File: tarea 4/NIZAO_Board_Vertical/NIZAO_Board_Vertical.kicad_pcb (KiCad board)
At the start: 2 copper layers, 36.2 x 39.5 mm, 3 parts

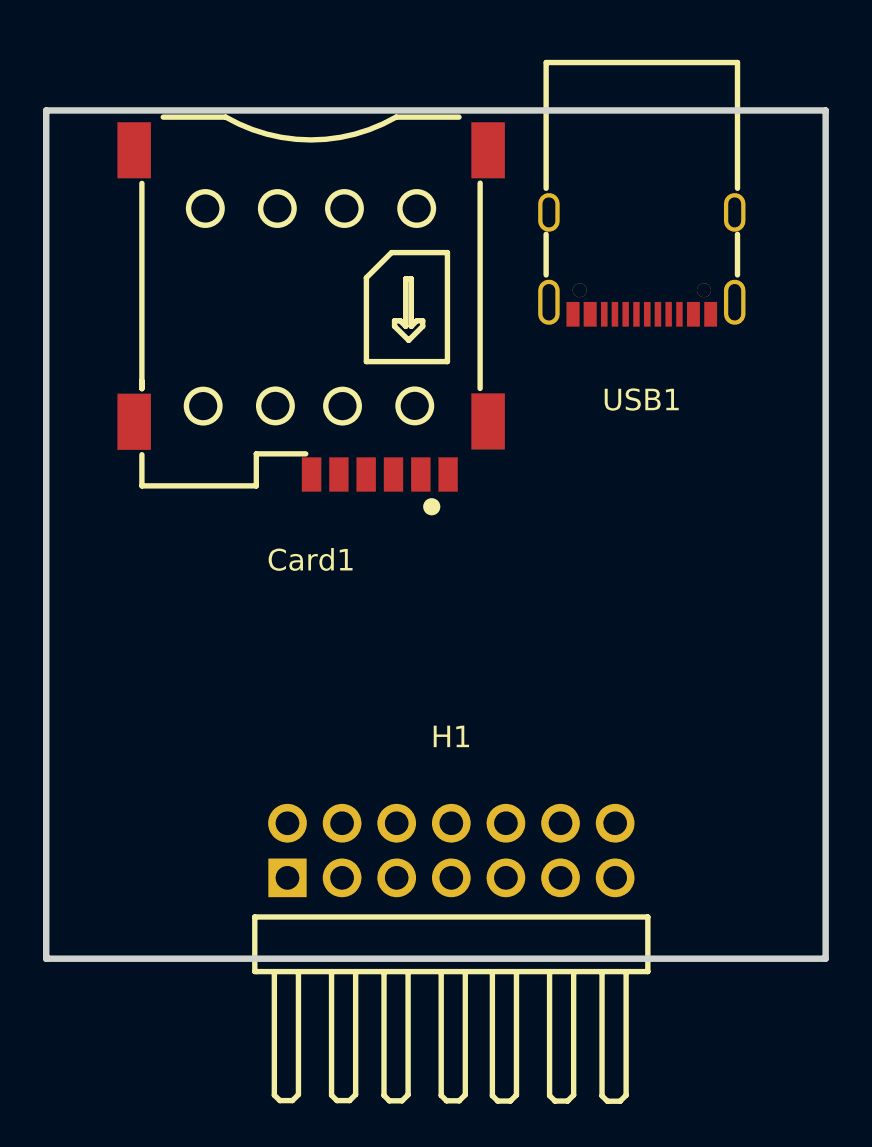
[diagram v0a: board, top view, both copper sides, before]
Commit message: actualizacion
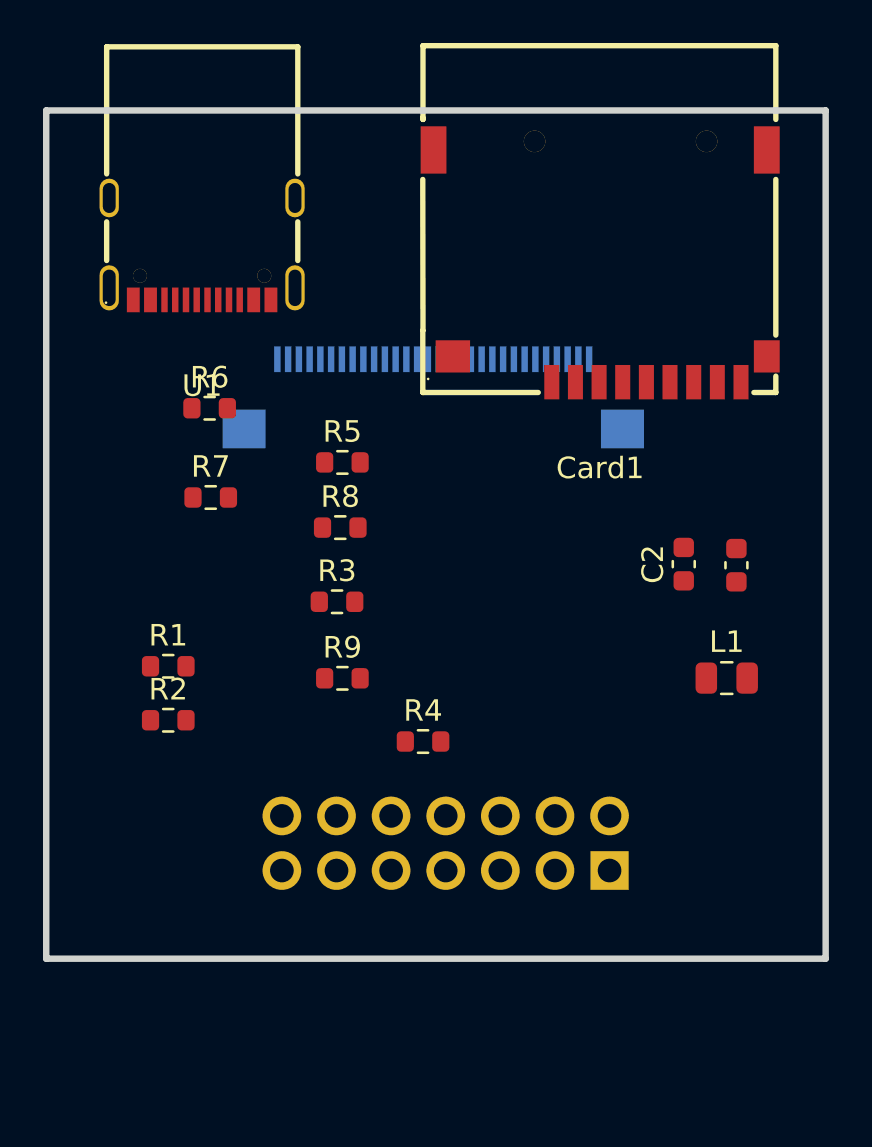
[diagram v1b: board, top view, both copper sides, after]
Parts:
- removed H1: PZ254R-12-14P, easyeda2kicad:HDR-TH_14P-P2.54-H-M-R2-C7-S2.54
- removed USB1: LCK-TCF809-L117YL-G1, easyeda2kicad:USB-C-SMD_LCK-TCF809-L117YL-G1
- added C1: 47uF, Capacitor_SMD:C_0603_1608Metric, F.Cu at (158.2, 102.2)
- added C2: 100nF, Capacitor_SMD:C_0603_1608Metric, F.Cu at (155.8, 102.1)
- added FPC1: FPC-05FB-30PH20, EasyEDA:FPC-SMD_30P-P0.50_FPC-05FB-30PH20, B.Cu at (144.1, 94.2)
- added J1: PZ254R-12-14P, EasyEDA:HDR-TH_14P-P2.54-H-M-R2-C7-S2.54, B.Cu at (144.7, 115.1)
- added L1: 600 Ohm, Capacitor_SMD:C_0805_2012Metric, F.Cu at (157.8, 107.4)
- added R1: 5.1k, Resistor_SMD:R_0603_1608Metric, F.Cu at (131.8, 106.8)
- added R2: 5.1k, Resistor_SMD:R_0603_1608Metric, F.Cu at (131.8, 109.4)
- added R3: 10K, Resistor_SMD:R_0603_1608Metric, F.Cu at (139.6, 103.8)
- added R4: 2.2K, Resistor_SMD:R_0603_1608Metric, F.Cu at (143.6, 110.3)
- added R5: 2.2K, Resistor_SMD:R_0603_1608Metric, F.Cu at (139.9, 97.4)
- added R6: 10R, Resistor_SMD:R_0603_1608Metric, F.Cu at (133.7, 94.8)
- added R7: 220R, Resistor_SMD:R_0603_1608Metric, F.Cu at (133.8, 99.0)
- added R8: 2.2K, Resistor_SMD:R_0603_1608Metric, F.Cu at (139.8, 100.4)
- added R9: 10K, Resistor_SMD:R_0603_1608Metric, F.Cu at (139.9, 107.4)
- added U1: MC-121-L119, EasyEDA:USB-C-SMD_HANBO_MC-121-L119, F.Cu at (133.3, 87.4)
- Card1: value SMC-202-6 -> TF-115; footprint easyeda2kicad:SIM-SMD_SMC-202-6 -> EasyEDA:TF-SMD_TF-115
- moved Card1 13.6 mm to (151.9, 88.2)
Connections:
- Card1 pad 10: unconnected-(Card1-GND-Pad10) -> GND
- Card1 pad 7: unconnected-(Card1-GND-Pad7) -> Net-(Card1-DAT0)
- Card1 pad 8: unconnected-(Card1-GND-Pad8) -> Net-(Card1-DAT1)
